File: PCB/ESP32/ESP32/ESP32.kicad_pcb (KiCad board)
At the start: 2 copper layers, 51 x 51 mm, 40 parts, among them J1 PPTC091LFBN-RC, J2 PPTC091LFBN-RC, U2 ESP32-S2-SOLO-U-N4

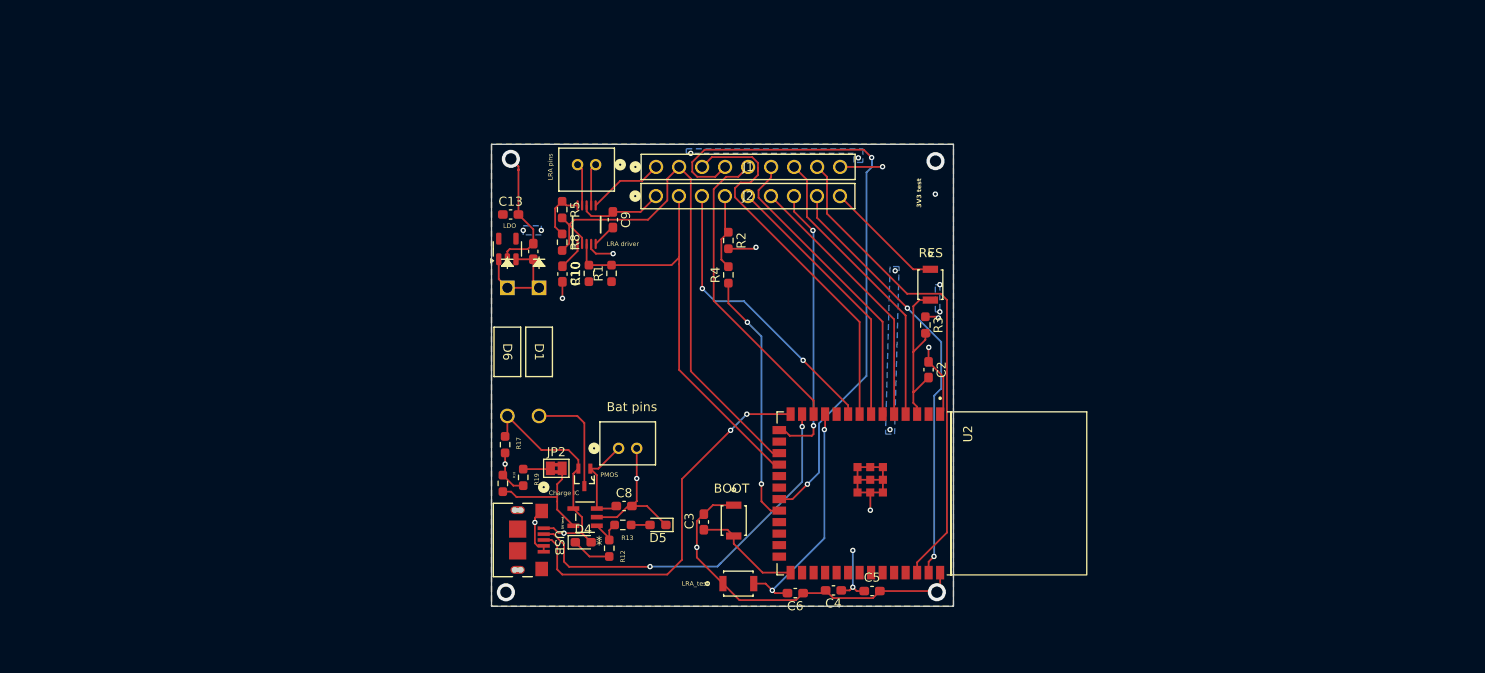
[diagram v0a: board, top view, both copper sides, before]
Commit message: WIP of the new layout.
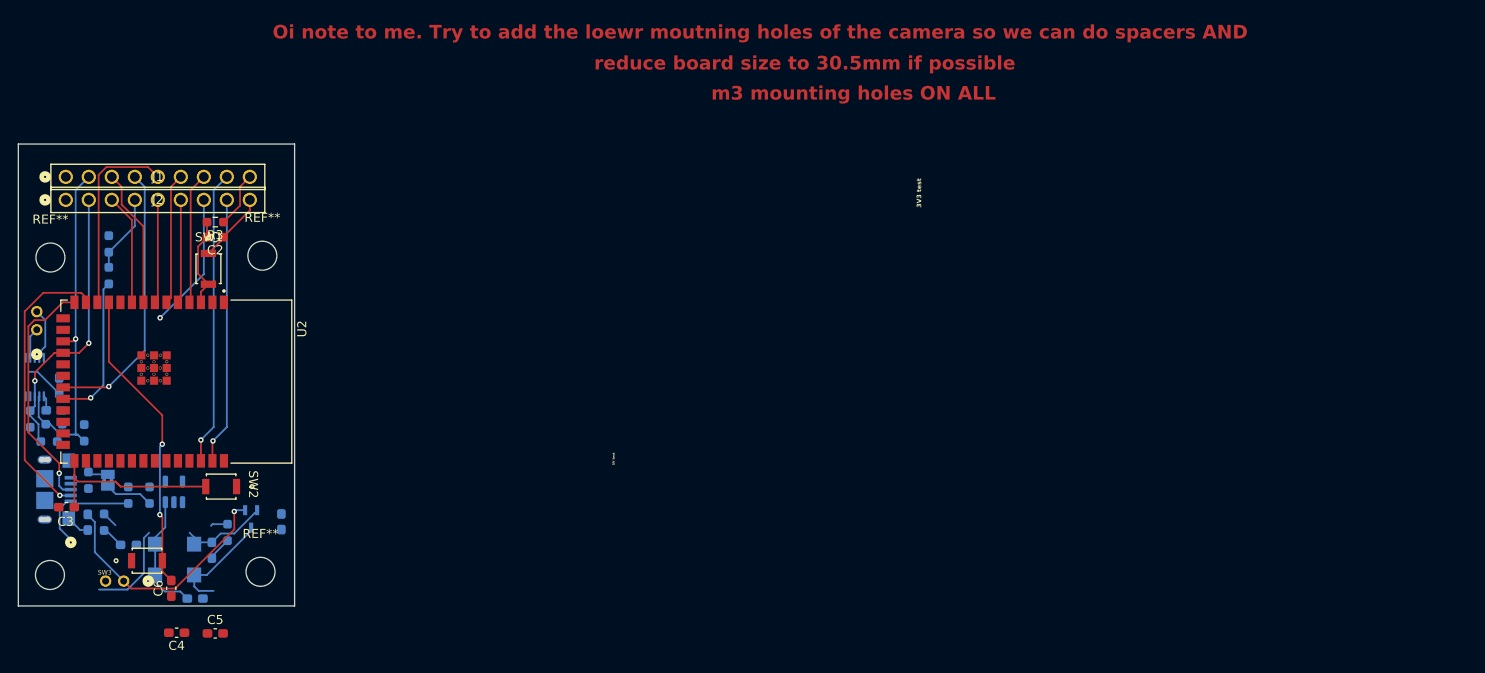
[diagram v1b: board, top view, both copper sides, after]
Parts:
- removed Charge IC: MCP73832T-2ACI/OT, Footprint:SOT-23-5_MC_MCH
- added REF**: MountingHole_3.2mm_M3, MountingHole:MountingHole_3.2mm_M3, F.Cu at (138.5, 147.7)
- added REF**: MountingHole_3.2mm_M3, MountingHole:MountingHole_3.2mm_M3, F.Cu at (115.2, 148.1)
- added REF**: MountingHole_3.2mm_M3, MountingHole:MountingHole_3.2mm_M3, F.Cu at (115.3, 113.0)
- added REF**: MountingHole_3.2mm_M3, MountingHole:MountingHole_3.2mm_M3, F.Cu at (138.7, 112.8)
- C10, C12, C13, C8, C9, D4, D5, JP2, R1, R10, R12, R13, R17, R18, R19, R2, R4, R5, R8: moved to B.Cu
- D1, D6: footprint Footprint:DO-41_STM -> Schottky_Diode_Battery:CR_SMA_403AE_OSI-L; moved to B.Cu
- J3: renamed from LRA pins; moved to B.Cu
- J4: renamed from Bat pins; moved to B.Cu
- J5: renamed from USB; moved to B.Cu
- Q1: renamed from PMOS; moved to B.Cu
- U2: footprint Footprint:XCVR_ESP32-S2-SOLO-U-N4 -> ESP32_sym_footprint:XCVR_ESP32-S2-SOLO-N4
- U5: renamed from LRA driver; moved to B.Cu
- U6: renamed from LDO; moved to B.Cu
- moved C2 80.1 mm to (133.5, 110.8), turned to 180 degrees
- moved SW1 79.7 mm to (132.8, 114.2)
- moved R3 79.2 mm to (133.5, 109.1), turned to 180 degrees
- moved U2 76.9 mm to (129.2, 126.7)
- moved C4 72.7 mm to (129.2, 154.4)
- moved C5 72.7 mm to (133.5, 154.5)
- moved C3 70.4 mm to (117.1, 140.6), turned to 0 degrees
- moved C6 68.9 mm to (128.7, 149.5), turned to 90 degrees
- moved R2 68.4 mm to (121.8, 111.5), turned to 90 degrees
- moved R4 68.4 mm to (121.8, 115.0)
- moved SW3 65.3 mm to (126.0, 146.5)
- moved J1 65.2 mm to (117.0, 104.1)
- moved J2 65.2 mm to (117.0, 106.6)
- moved R1 64.8 mm to (115.2, 133.3), turned to 180 degrees
- moved J3 64.3 mm to (113.8, 121.0), turned to -90 degrees
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- renumbered RES to SW1, BOOT to SW2, LRA_test to SW3
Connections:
- net 5V renamed Net-(D4-A)
- net Charge-line renamed Net-(J4-Pin_1)
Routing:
- net GND: track 137.4 -> 11.3 mm, vias 13 -> 0
- net /PCLK: track 68.9 -> 30.3 mm, vias 2 -> 1
- net /VS: track 42.3 -> 15.3 mm
- net /D1: track 54.3 -> 32.5 mm, vias 0 -> 1
- net +3V3: track 27.7 -> 6.19 mm, vias 13 -> 0
- net /SCL: track 59.7 -> 39.1 mm, vias 0 -> 1
- net /HS: track 32.6 -> 12.2 mm, vias 2 -> 0
- net /D5: track 33.5 -> 14.5 mm
- net /D0: track 47.8 -> 29.5 mm, vias 2 -> 1
- net /D6: track 29.7 -> 11.4 mm
- net /D4: track 29.7 -> 11.4 mm
- net /D3: track 32.4 -> 14.5 mm
- net /USB_D+: track 42.9 -> 26.7 mm, vias 2 -> 1
- net /D2: track 31.2 -> 15.1 mm, vias 2 -> 1
- net Net-(J4-Pin_1): track 11.4 -> 27.4 mm, vias 0 -> 1
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- removed copper zone on B.Cu, net +3V3
- removed copper zone on F.Cu, net +3V3
- removed copper zone on B.Cu, net GND
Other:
- board size 51 x 51 mm -> 30.5 x 51 mm
- board text added: "Boot Switch"
- board text added: "Oi note to me. Try to add the loewr moutning holes of the camera so we can do spacers AND"
- board text added: "m3 mounting holes ON ALL"
- board text added: "reduce board size to 30.5mm if possible"
